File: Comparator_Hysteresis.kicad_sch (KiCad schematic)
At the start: 9 parts, among them U8 LMH6611

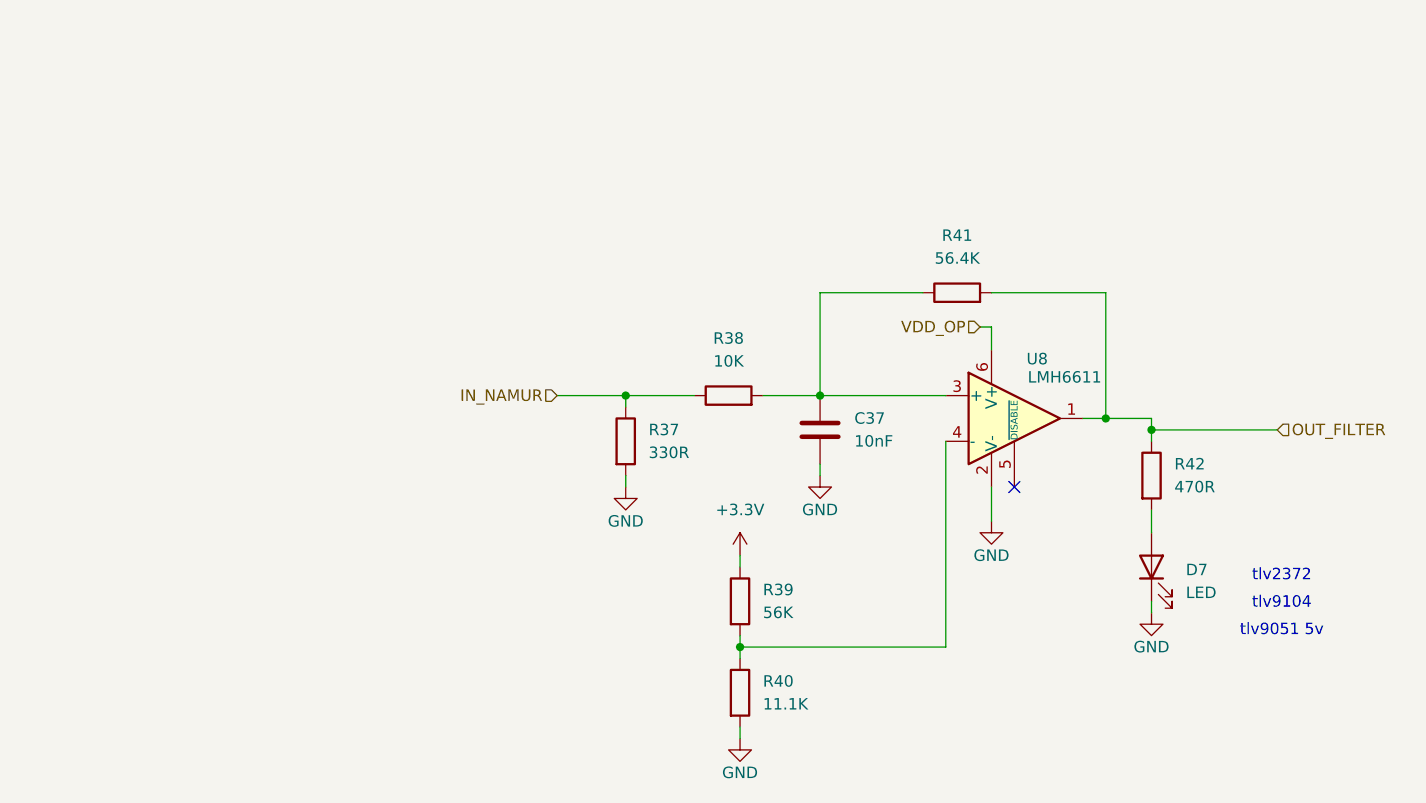
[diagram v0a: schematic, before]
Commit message: Avance
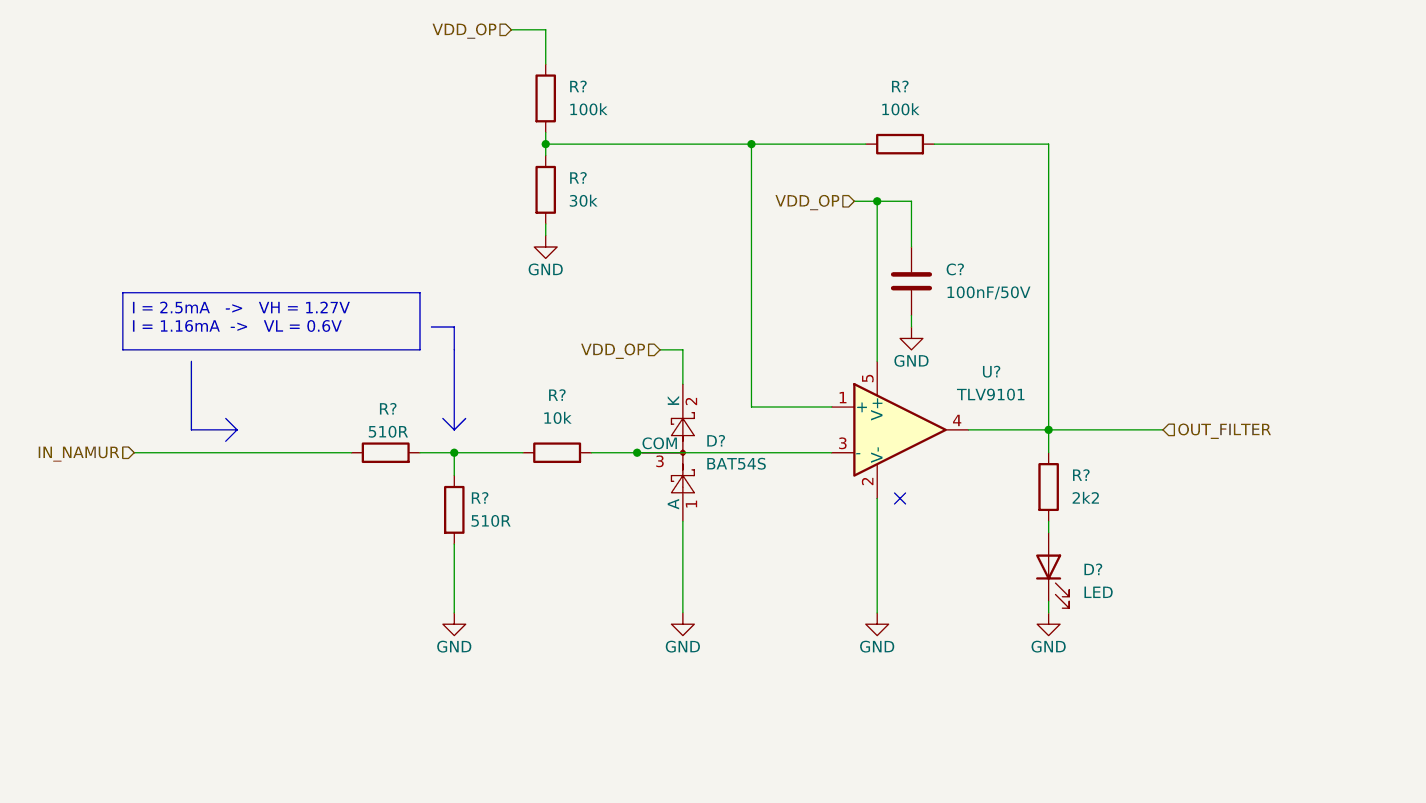
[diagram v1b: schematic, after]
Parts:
- removed U8: LMH6611, Package_TO_SOT_SMD:TSOT-23-6, symbol Amplifier_Operational:LMH6611
- added D?: BAT54S, Package_TO_SOT_SMD:SOT-23, symbol Diode:BAT54S
- added R?: 10k, symbol 1-Resistor:R
- added U?: TLV9101, LIB_PCB_CONT:SC70-5_TexasInstruments, symbol LIB_SCH_CONTR:TLV9101
- C?: renamed from C37; value 10nF -> 100nF/50V
- R?: renamed from R40; value 11.1K -> 30k
- R?: renamed from R37; value 330R -> 510R
- R?: renamed from R41; value 56.4K -> 100k
- R?: renamed from R39; value 56K -> 100k
- R?: renamed from R38; value 10K -> 510R
- R?: renamed from R42; value 470R -> 2k2
- renumbered D7 to D?
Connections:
- net +3.3V is gone; now on net VDD_OP: R?.1
- net GND: now also D?.1 (A), U?.2 (V-)
- net IN_NAMUR: no longer R?.1
- net OUT_FILTER: now also U?.4
- net VDD_OP: now also C?.1, D?.2 (K), U?.5 (V+)
- net at R?.1, R?.2: now also R?.1, U?.1 (+)
- new net: D?.3 (COM), R?.2, U?.3 (-)
- new net: R?.1, R?.1, R?.2
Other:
- note removed: "tlv2372"
- note removed: "tlv9051 5v"
- note removed: "tlv9104"
- moved on the sheet: C?, D?, R?
